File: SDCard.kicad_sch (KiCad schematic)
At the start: 5 parts, among them J7 Micro_SD_Card_Det, U22 RT9742GGJ5

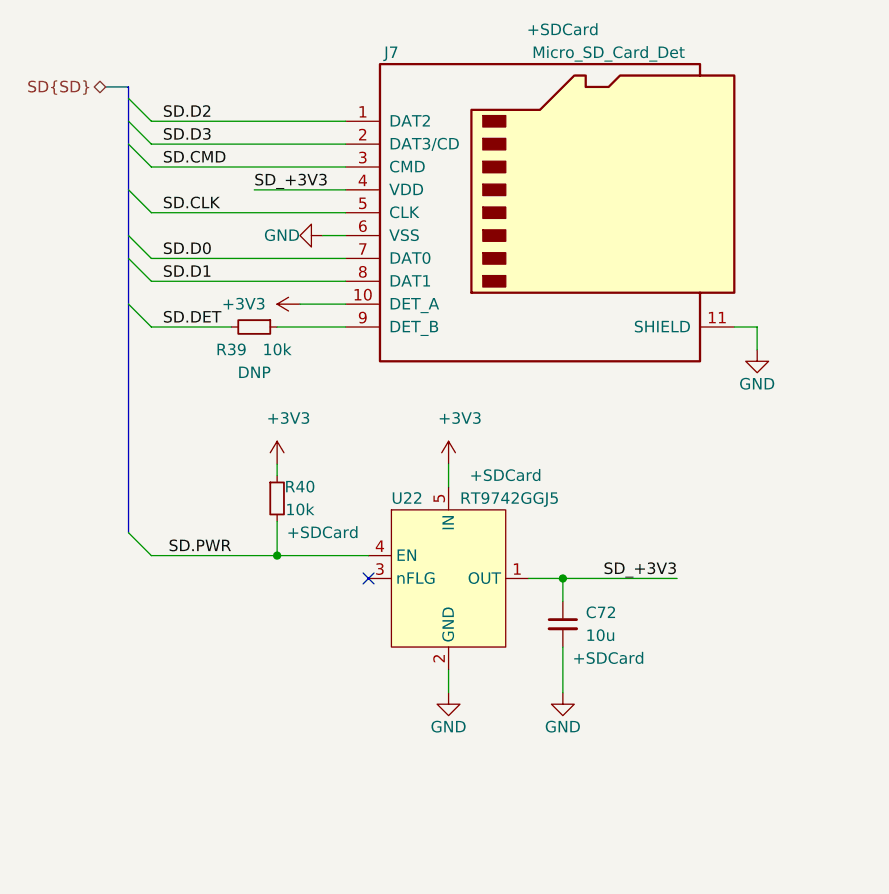
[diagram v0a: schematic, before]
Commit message: Weeded out all ERC errors
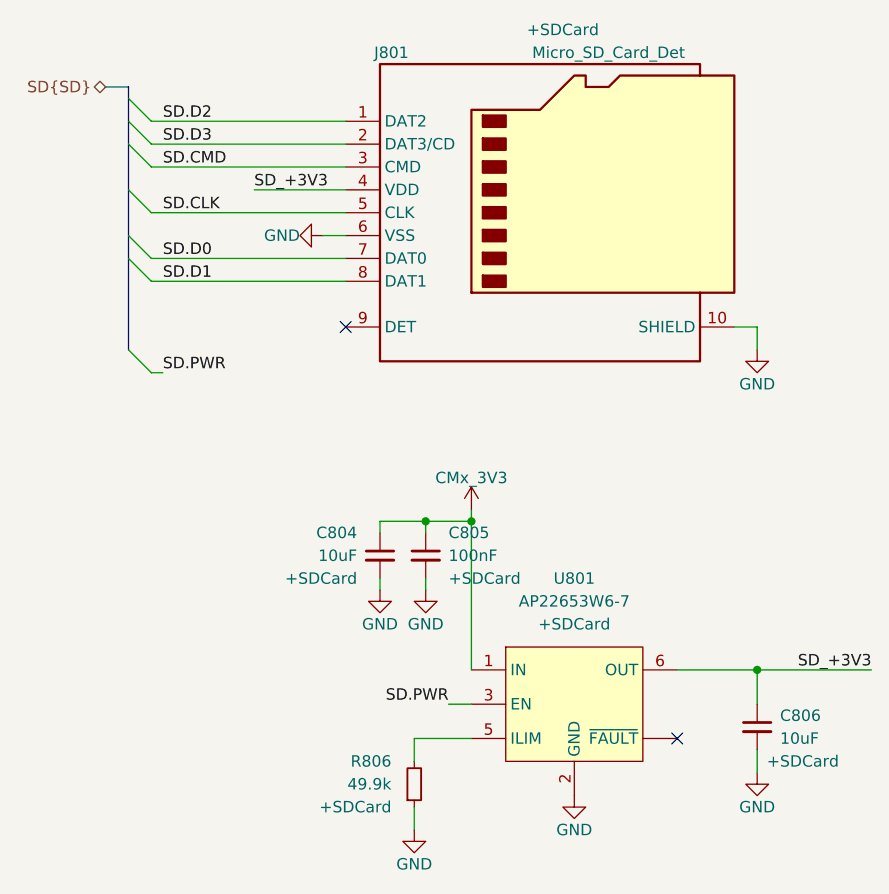
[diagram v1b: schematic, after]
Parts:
- removed C72: 10u, Capacitor_SMD:C_0805_2012Metric, symbol Device:C_Small
- removed R39, R40: 10k, Resistor_SMD:R_0402_1005Metric, symbol Device:R_Small
- removed U22: RT9742GGJ5, Package_TO_SOT_SMD:SOT-23-5, symbol Yellow:RT9742GGJ5
- added C804, C806: 10uF, Capacitor_SMD:C_0805_2012Metric, symbol Device:C_Small
- added C805: 100nF, Capacitor_SMD:C_0402_1005Metric, symbol Device:C_Small
- added R806: 49.9k, Resistor_SMD:R_0603_1608Metric, symbol Device:R_Small
- added U801: AP22653W6-7, Package_TO_SOT_SMD:SOT-23-6, symbol Hatlabs:AP22653
- J801: renamed from J7; footprint Connector_Card:microSD_HC_Molex_104031-0811 -> Hatlabs:MicroSD_SHOU-HAN_TF-PUSH; symbol Connector:Micro_SD_Card_Det -> Connector:Micro_SD_Card_Det1; LCSC (none) -> C393941; Manufacturer Molex -> SHOU HAN; PartNumber 104031-0811 -> TF PUSH
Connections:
- net +3V3 is gone; now on net GND: J801.10 (SHIELD)
- net GND: now also C804.2, C805.2, C806.2, R806.1, U801.2 (GND); no longer J801.11 (SHIELD)
- net SD.PWR: now also U801.3 (EN)
- net SD_+3V3: now also C806.1, U801.6 (OUT)
- new net: R806.2, U801.5 (ILIM)
- new net CMx_3V3: C804.1, C805.1, U801.1 (IN)
- no-connect marks 1 -> 2
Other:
- company: Nabu Casa -> Hat Labs Oy
- title: SD card -> HALPI2
